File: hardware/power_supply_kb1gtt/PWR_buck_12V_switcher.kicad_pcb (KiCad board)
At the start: 2 copper layers, 38.1 x 38.7 mm, 22 parts, among them P1 CONN_2, P2 CONN_1, P3 CONN_2, P4 CONN_1, Q1 30V, Q2 200V, U1 LM2596

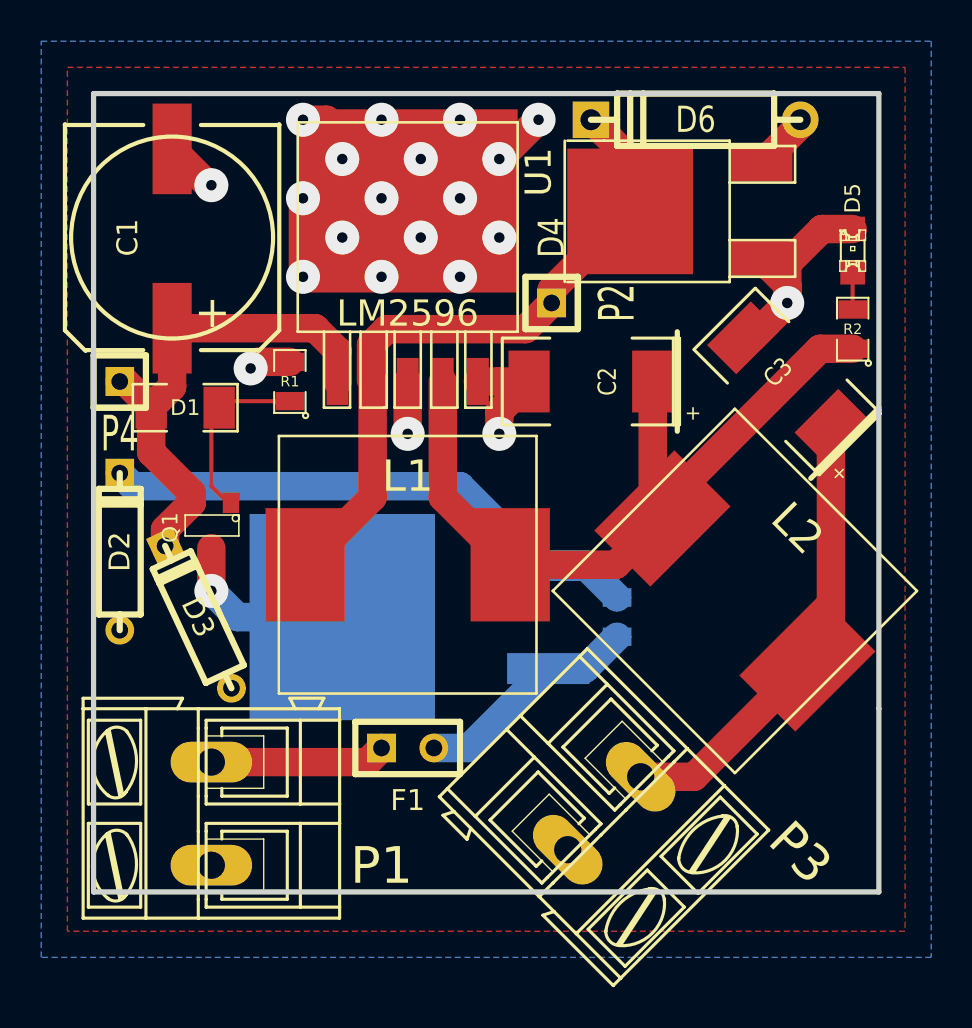
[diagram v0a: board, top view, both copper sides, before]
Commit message: auto-sync
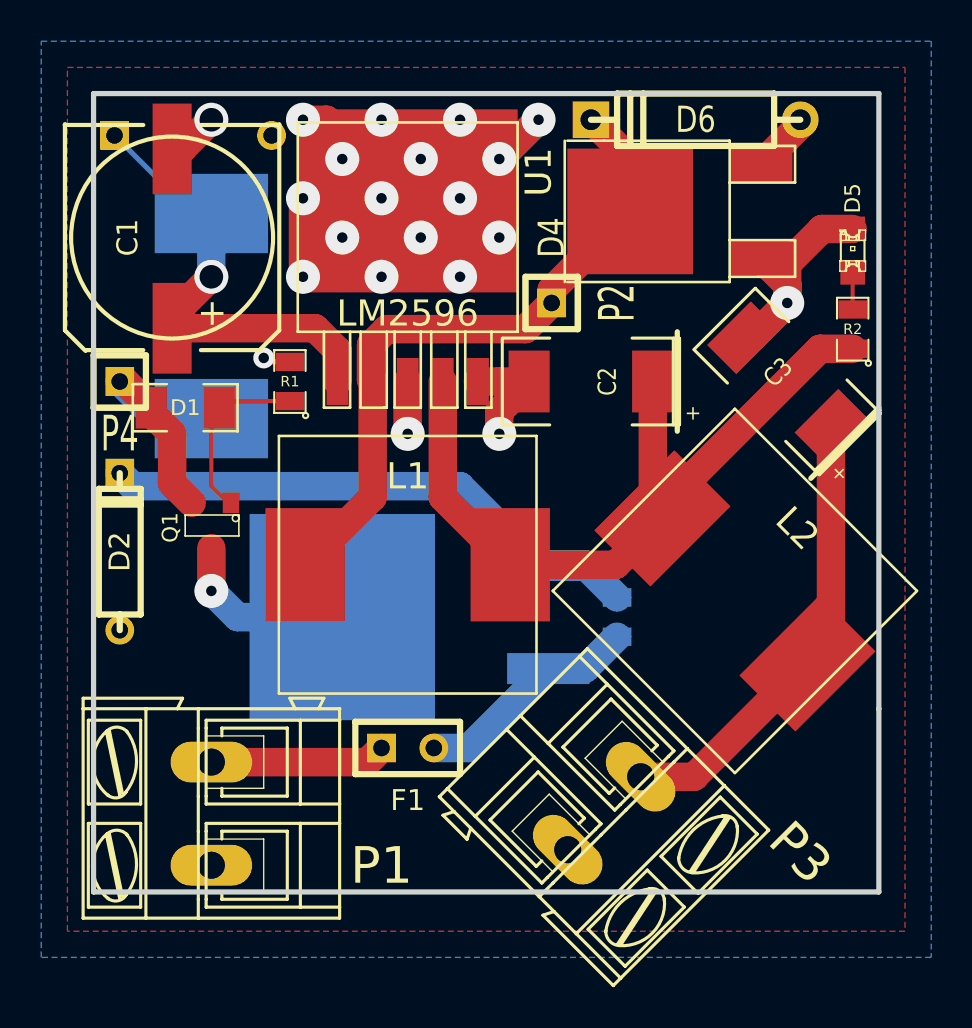
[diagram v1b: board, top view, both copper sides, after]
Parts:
- added L3: 38uH, SM100uH, B.Cu at (168.3, 106.0)
- D2: value 15V -> 14V
- D3: moved to B.Cu
- Q1: value 30V -> 20V
- moved D3 23.4 mm to (167.4, 97.3), turned to 180 degrees
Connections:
- D1 pad 2: /VBAT -> Net-(D1-Pad2)
- P4 pad 1: /VBAT -> Net-(D1-Pad2)
- Q1 pad 2: /VBAT -> Net-(D1-Pad2)
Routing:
- net Net-(D1-Pad2): track 0.00 -> 12.7 mm
- net /VBAT: track 24.4 -> 22.6 mm, vias 0 -> 1
- net GND: track 83.0 -> 82.2 mm
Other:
- rule via_min_drill: 0.508 -> 0.3
